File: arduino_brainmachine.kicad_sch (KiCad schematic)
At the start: 66 parts, among them Q1 2N5551, Q2 2N5551, Q3 2N5551, Q4 2N5551, Q5 PNP, Q6 PNP, SW1 SW_Push, U1 VOS618A, U2 VOS618A

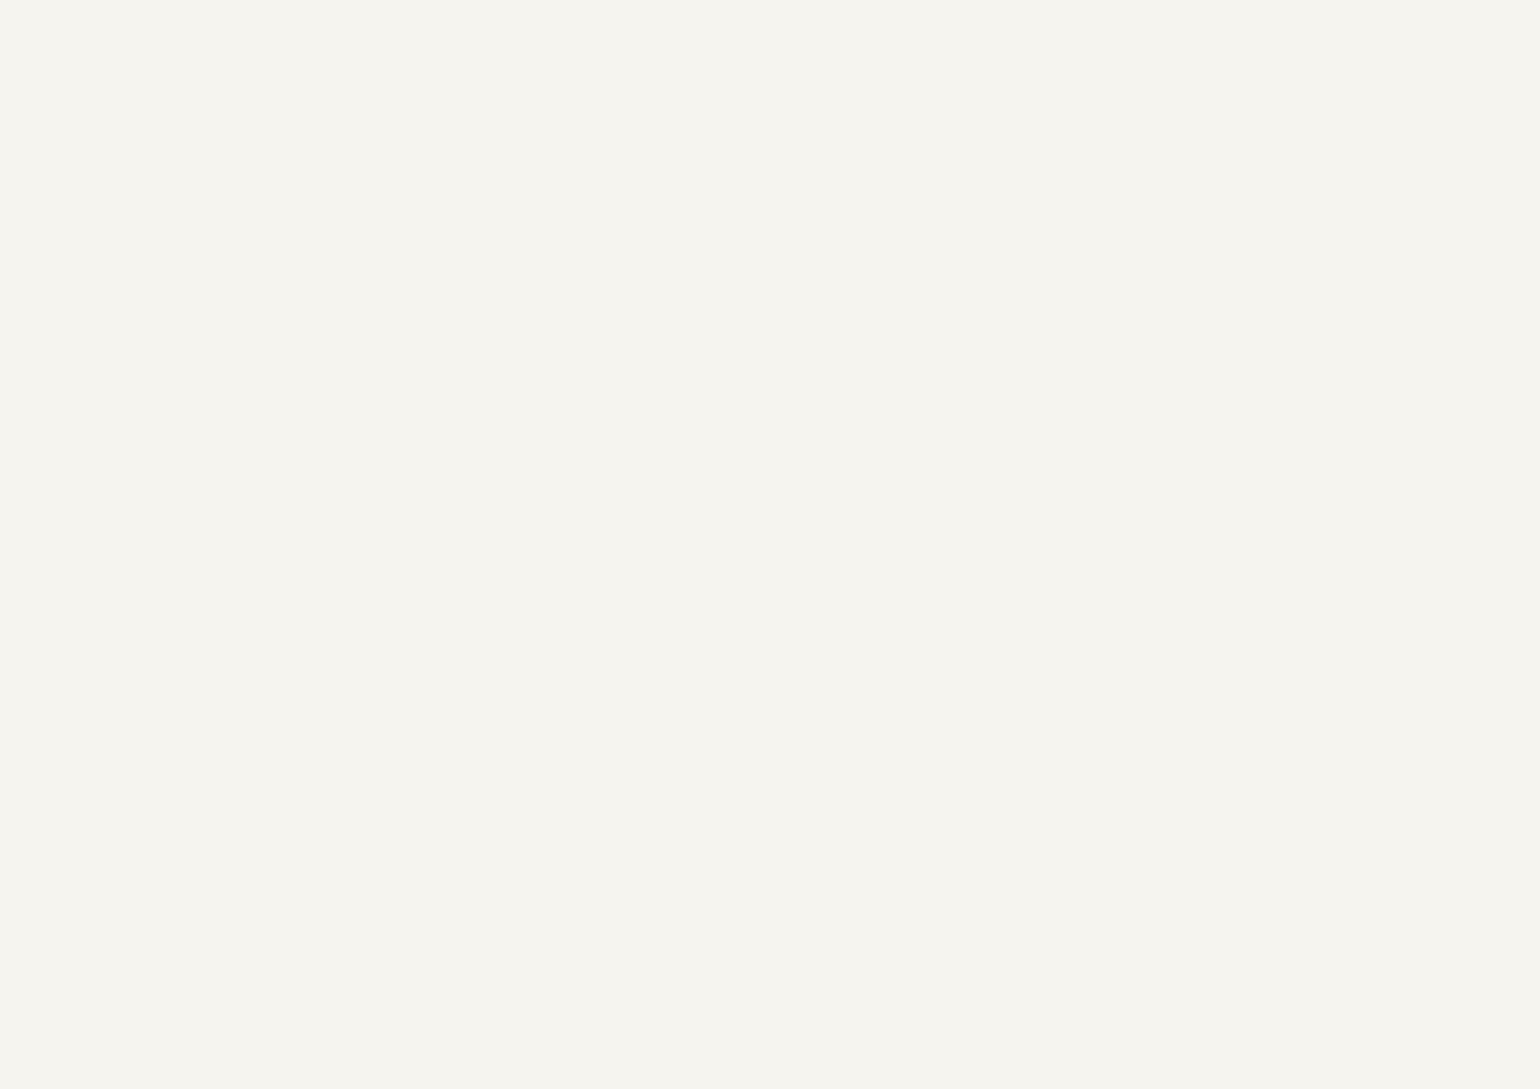
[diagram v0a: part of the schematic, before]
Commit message: Upgrade
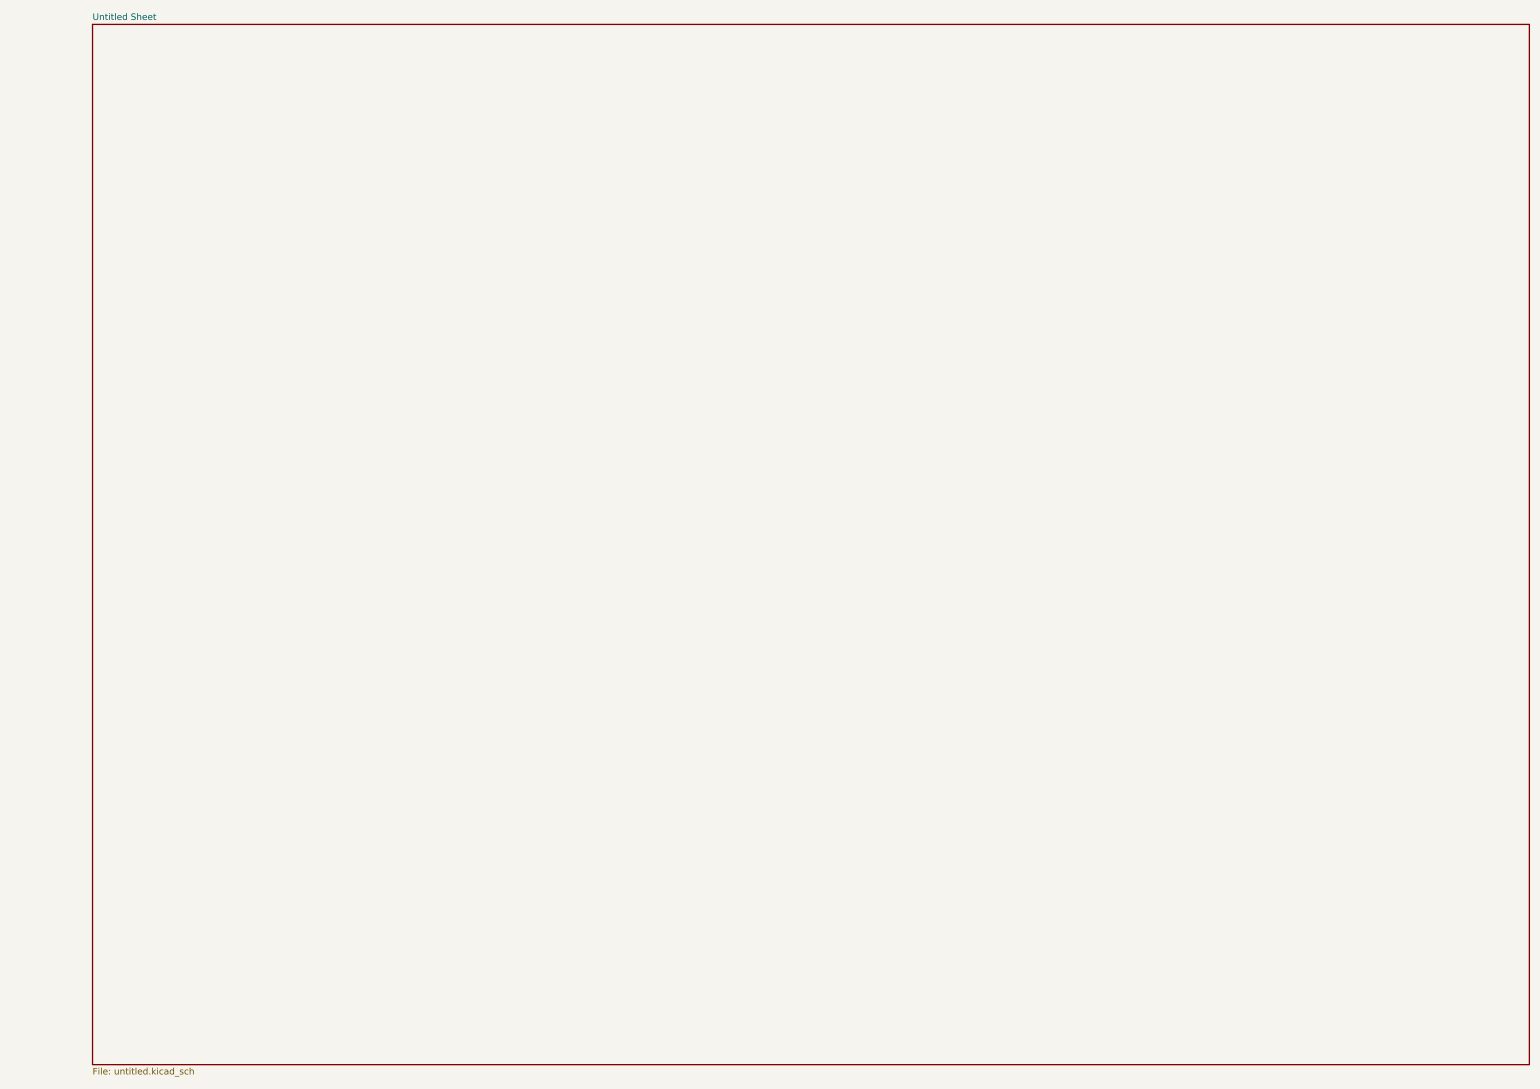
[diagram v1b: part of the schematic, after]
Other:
- added sheet Untitled Sheet (untitled.kicad_sch)
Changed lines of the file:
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@@
 	(generator_version "8.0")
 	(paper "A4")
+	(title_block
+		(date "2025-02-18")
+	)
 	(junction
 		(at 40.64 96.52)
@@
 		)
 	)
+	(sheet
+		(at 306.07 2.54)
+		(size 280.67 203.2)
+		(fields_autoplaced yes)
+		(stroke
+			(width 0.1524)
+			(type solid)
+		)
+		(fill
+			(color 0 0 0 0.0000)
+		)
+		(property "Sheetname" "Untitled Sheet"
+			(at 306.07 1.8284 0)
+			(effects
+				(font
+					(size 1.27 1.27)
+				)
+				(justify left bottom)
+			)
+		)
+		(property "Sheetfile" "untitled.kicad_sch"
+			(at 306.07 206.3246 0)
+			(effects
+				(font
+					(size 1.27 1.27)
+				)
+				(justify left top)
+			)
+		)
+		(instances
+			(project "arduino_brainmachine"
+				(path "/16427a71-30ca-4ef8-b47f-54137aef95d2"
+					(page "2")
+				)
+			)
+		)
+	)
 	(sheet_instances
 		(path "/"
-			(page "1")
+			(page "2")
 		)
 	)

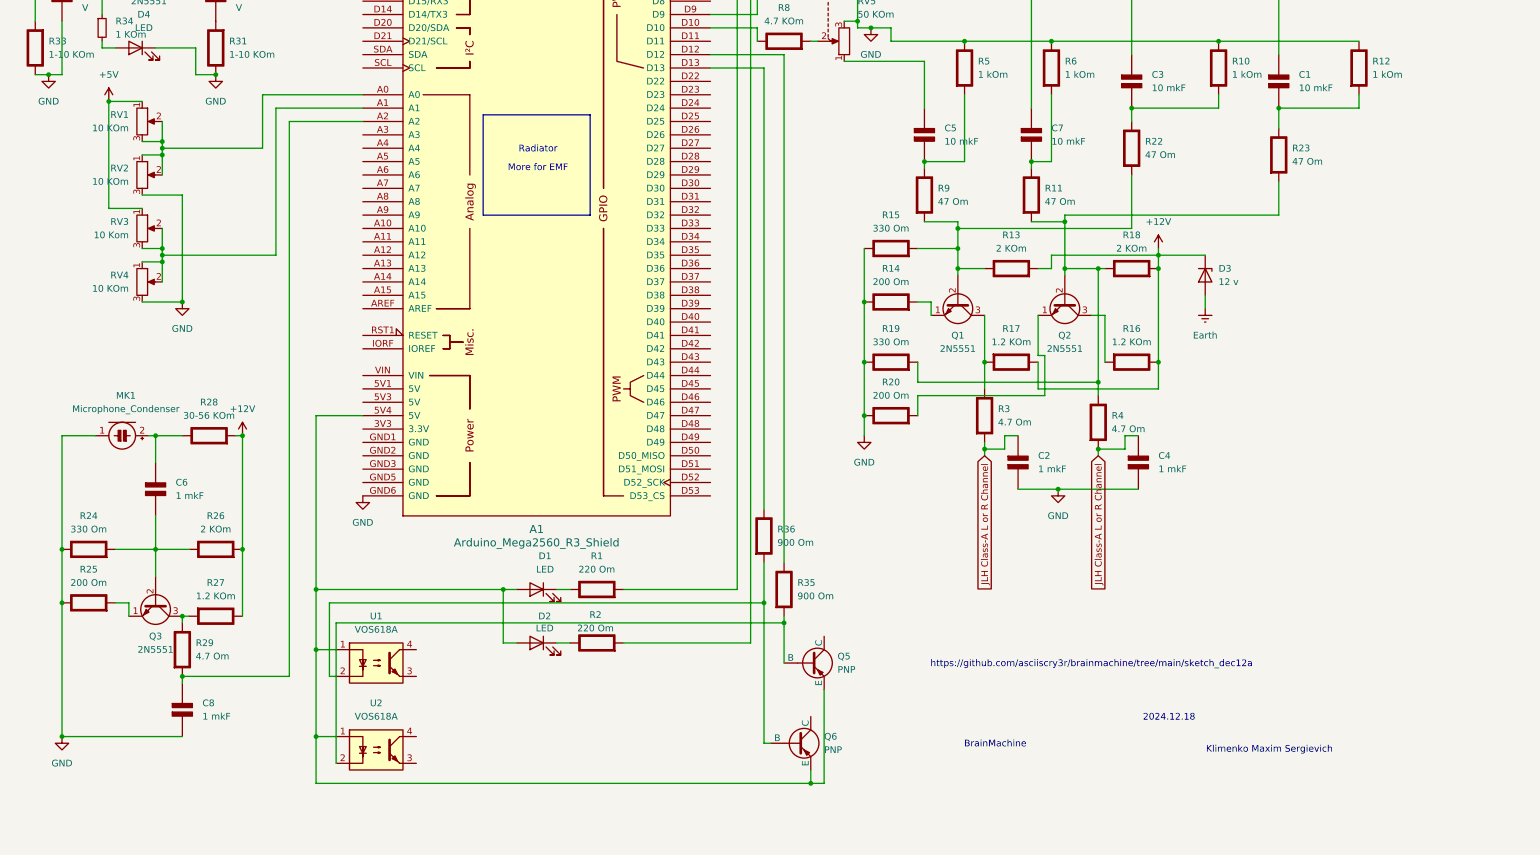
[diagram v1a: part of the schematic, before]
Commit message: Upgarde
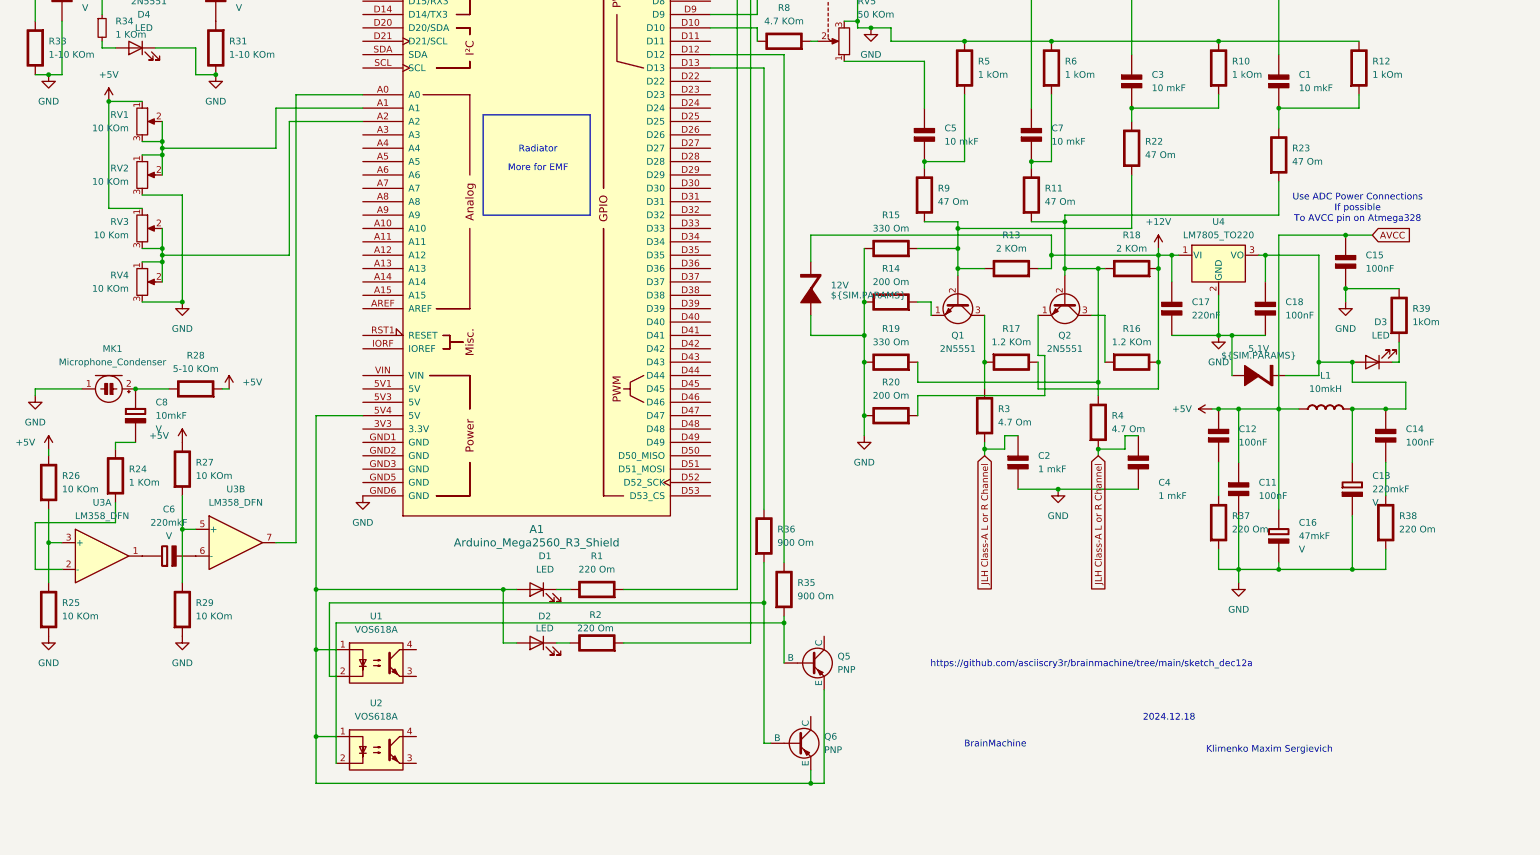
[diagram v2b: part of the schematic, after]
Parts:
- removed C6, C8: 1 mkF, symbol PCM_Elektuur:C
- removed D3: 12 v, symbol Device:D_Zener
- removed Q3: 2N5551, Package_TO_SOT_THT:TO-39-3, symbol Transistor_BJT:2N2219
- added 12V, 5.1V: ${SIM.PARAMS}, symbol PCM_Elektuur:D-Zener
- added C11, C12, C14, C15, C18: 100nF, symbol PCM_Elektuur:C
- added C13, C6: 220mkF, symbol PCM_Elektuur:C-polar
- added C16: 47mkF, symbol PCM_Elektuur:C-polar
- added C17: 220nF, symbol PCM_Elektuur:C
- added C8: 10mkF, symbol PCM_Elektuur:C-polar
- added D3: LED, symbol Device:LED
- added L1: 10mkH, symbol PCM_Elektuur:L
- added R37, R38: 220 Om, symbol PCM_Elektuur:R
- added R39: 1kOm, symbol PCM_Elektuur:R
- added U3: LM358_DFN, Package_DFN_QFN:DFN-8-1EP_2x2mm_P0.5mm_EP1.05x1.75mm, symbol Amplifier_Operational:LM358_DFN
- added U4: LM7805_TO220, Package_TO_SOT_THT:TO-220-3_Vertical, symbol Regulator_Linear:LM7805_TO220
- R24: value 330 Om -> 1 KOm
- R25: value 200 Om -> 10 KOm
- R26: value 2 KOm -> 10 KOm
- R27: value 1.2 KOm -> 10 KOm
- R28: value 30-56 KOm -> 5-10 KOm
- R29: value 4.7 Om -> 10 KOm
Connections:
- net +12V: now also 12V.1 (K-), C17.1 (+), U4.1 (VI); no longer R26.2 (-), R27.1 (+), R28.2 (-)
- net +5V: now also R26.1 (+), R27.1 (+), R28.2 (-), C11.1 (+), C12.1 (+), C15.1 (+), C16.1 (+), L1.1 (+)
- net GND: now also R25.2 (-), R29.2 (-), 12V.2 (A+), 5.1V.2 (A+), C11.2 (-), C13.2 (-), C15.2 (-), C16.2 (-), C17.2 (-), C18.2 (-), R37.2 (-), R38.2 (-), R39.1 (+), U4.2 (GND); no longer R24.1 (+), R25.1 (+)
- net at MK1.2 (+), R28.1 (+): now also C8.1 (+)
- net at R24.2 (-): now also U3.2 (-); no longer R26.1 (+)
- net at RV1.2, RV1.3, RV2.1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: now also A1.A1; no longer A1.A0
- net at RV3.2, RV3.3, RV4.1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: now also A1.A2; no longer A1.A1
- net at R27.2 (-), R29.1 (+): now also U3.5 (+)
- new net: C12.2 (-), R37.1 (+)
- new net: 5.1V.1 (K-), C13.1 (+), C14.1 (+), C18.1 (+), D3.2 (A), L1.2 (-), U4.3 (VO)
- new net: A1.A0, U3.7
- new net: C6.2 (-), U3.6 (-)
- new net: C6.1 (+), U3.1
- new net: D3.1 (K), R39.2 (-)
- new net: C8.2 (-), R24.1 (+)
- new net: R25.1 (+), R26.2 (-), U3.3 (+)
- new net: C14.2 (-), R38.1 (+)
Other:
- note added: "Use ADC Power Connections If possible To AVCC pin on Atmega328"
- moved on the sheet: MK1, R28
